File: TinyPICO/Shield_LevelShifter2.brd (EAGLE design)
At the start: 31.9 x 17.8 mm, 15 parts, among them U4 SN74HCT245DBRDB20-M

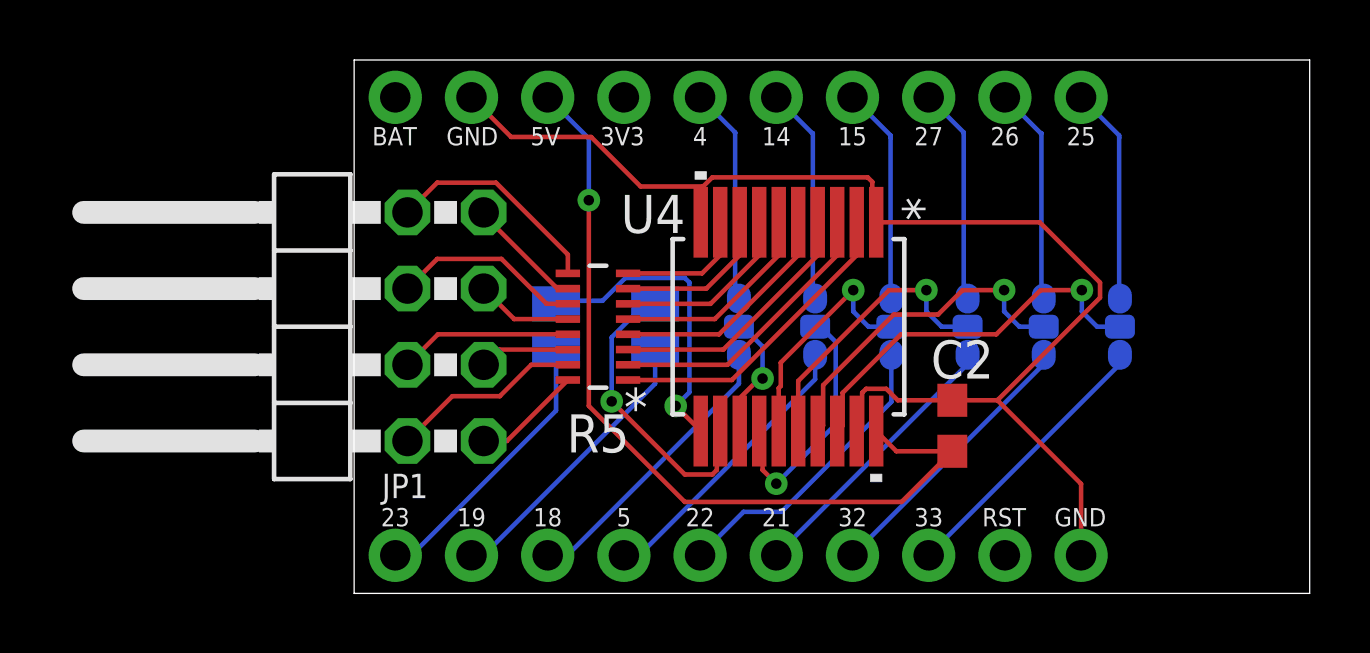
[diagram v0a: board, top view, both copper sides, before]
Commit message: Checkpoint
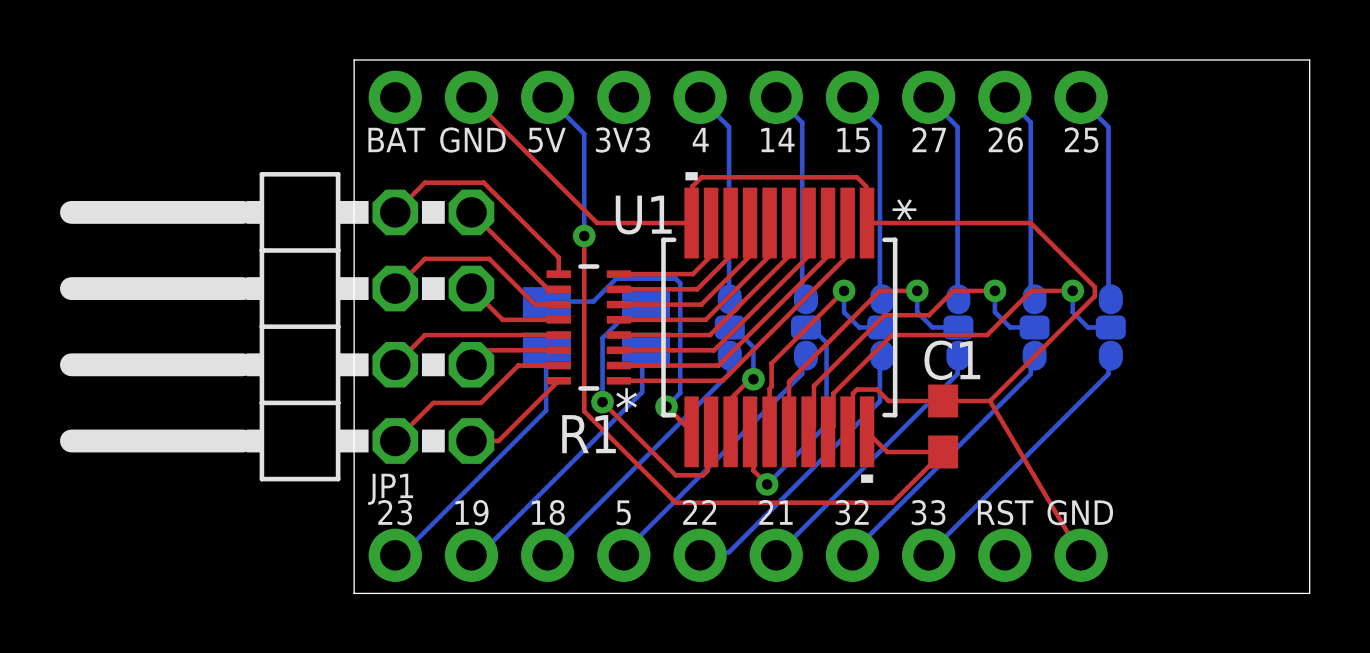
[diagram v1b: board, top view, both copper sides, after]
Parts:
- removed C2: 0.1uF, adafruit:C0603
- removed R5: EXB-2HV331JVEXB2HV-M, pv:EXB2HV-M
- removed U4: SN74HCT245DBRDB20-M, SN74HCT245:DB20-M
- added C1: 0.1uF, adafruit:C0603
- added R1: EXB-2HV331JVEXB2HV-M, pv:EXB2HV-M
- added U1: SN74HCT245DBRDB20-M, SN74HCT245:DB20-M
- moved JP1 0.41 mm to (-2.44, 8.89)
- moved 1 0.31 mm to (25.2, 8.86)
- moved 3 0.31 mm to (20.1, 8.86)
- moved 4 0.31 mm to (17.6, 8.86)
- moved 5 0.31 mm to (15.1, 8.86)
- moved 6 0.31 mm to (12.5, 8.86)
- moved 7 0.31 mm to (9.73, 8.86)
- moved 8 0.31 mm to (6.43, 8.86)
- moved 2 0.31 mm to (22.7, 8.86)
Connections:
- net 5V: now also C1.1, U1.20; no longer C2.1, U4.20
- net A1: now also R1.1, U1.2; no longer R5.1, U4.2
- net A2: now also R1.2, U1.3; no longer R5.2, U4.3
- net A3: now also R1.3, U1.4; no longer R5.3, U4.4
- net A4: now also R1.4, U1.5; no longer R5.4, U4.5
- net A5: now also R1.5, U1.6; no longer R5.5, U4.6
- net A6: now also R1.6, U1.7; no longer R5.6, U4.7
- net A7: now also R1.7, U1.8; no longer R5.7, U4.8
- net A8: now also R1.8, U1.9; no longer R5.8, U4.9
- net B1: now also U1.18; no longer U4.18
- net B2: now also U1.17; no longer U4.17
- net B3: now also U1.16; no longer U4.16
- net B4: now also U1.15; no longer U4.15
- net B5: now also U1.14; no longer U4.14
- net B6: now also U1.13; no longer U4.13
- net B7: now also U1.12; no longer U4.12
- net B8: now also U1.11; no longer U4.11
- net GND: now also C1.2, U1.1, U1.10, U1.19; no longer C2.2, U4.1, U4.10, U4.19
- net N$1: now also R1.16; no longer R5.16
- net N$2: now also R1.13; no longer R5.13
- net N$3: now also R1.15; no longer R5.15
- net N$4: now also R1.14; no longer R5.14
- net N$5: now also R1.12; no longer R5.12
- net N$6: now also R1.11; no longer R5.11
- net N$7: now also R1.10; no longer R5.10
- net N$8: now also R1.9; no longer R5.9
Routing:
- net GPIO18: track 9.71 -> 9.18 mm
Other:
- board text added: "LevelShifter 2.3"
- board text added: "http://swooby.com/PCBTP"
- board text removed: "LEVEL SHIFTER 2.0"
- board text removed: "https://github.com/swooby/pcb/tree/master/TinyPICO"
